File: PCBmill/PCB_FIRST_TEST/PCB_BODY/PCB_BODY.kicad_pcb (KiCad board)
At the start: 2 copper layers, 19 x 23.5 mm, 5 parts, among them U1 PC817

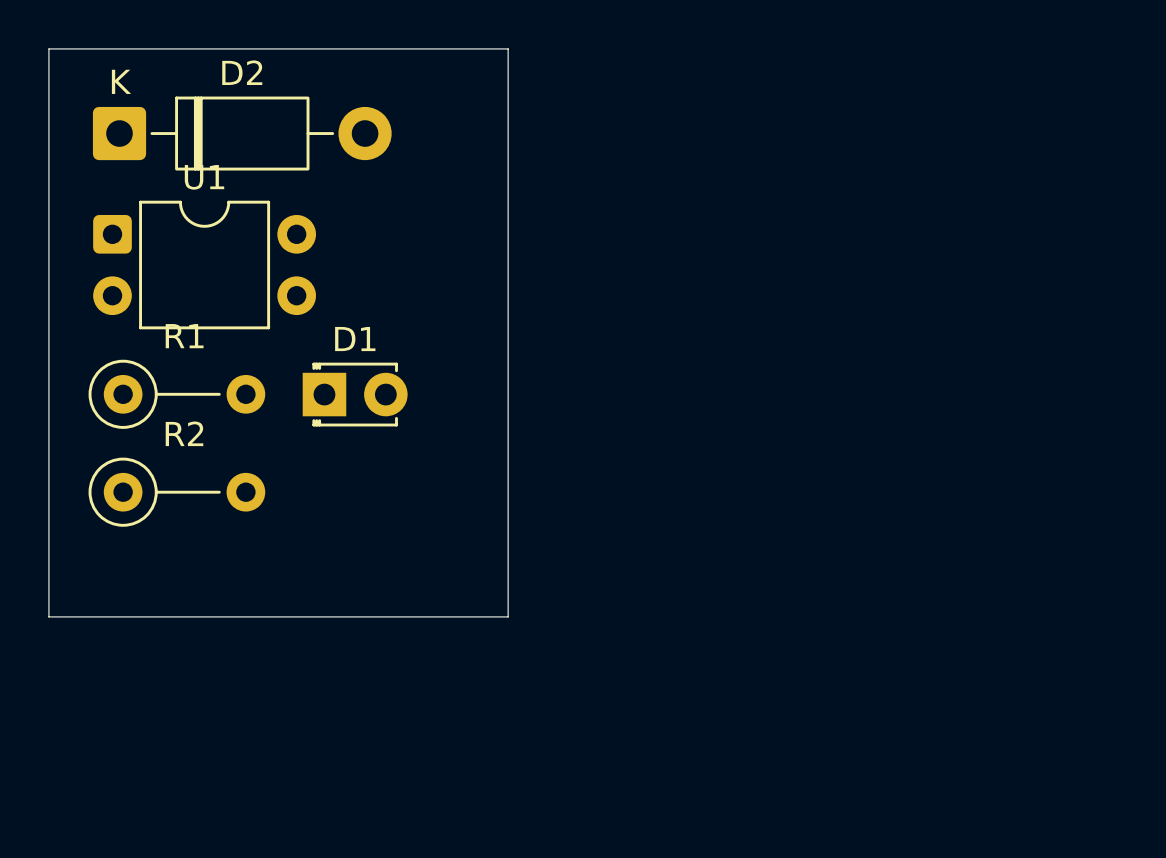
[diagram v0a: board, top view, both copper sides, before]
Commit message: added the thhings to the stuff
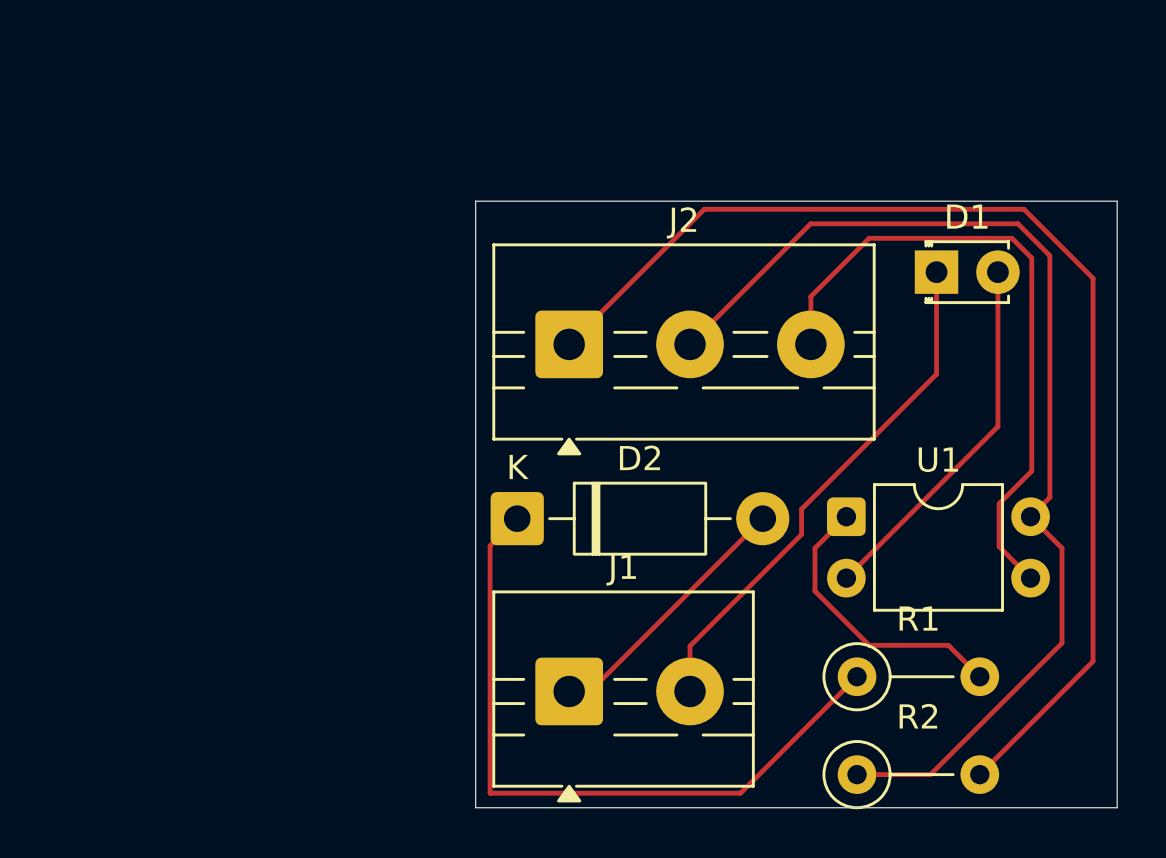
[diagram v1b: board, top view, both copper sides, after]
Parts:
- added J1: Screw_Terminal_01x02, TerminalBlock:TerminalBlock_MaiXu_MX126-5.0-02P_1x02_P5.00mm, F.Cu at (35.5, 41.1)
- added J2: Screw_Terminal_01x03, TerminalBlock:TerminalBlock_MaiXu_MX126-5.0-03P_1x03_P5.00mm, F.Cu at (35.5, 26.7)
- moved R1 32.5 mm to (47.4, 40.5)
- moved R2 32.5 mm to (47.4, 44.5)
- moved U1 32.5 mm to (47.0, 33.9)
- moved D1 25.8 mm to (50.7, 23.7)
- moved D2 22.9 mm to (33.4, 33.9)
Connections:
- D1 pad 1: GND -> Net-(D1-K)
- D2 pad 2: unconnected-(D2-A-Pad2) -> Net-(D2-A)
- R2 pad 2: +3.3V -> Net-(J2-Pin_1)
- U1 pad 1: Net-(D1-A) -> Net-(R1-Pad2)
- U1 pad 2: Net-(R1-Pad2) -> Net-(D1-A)
- U1 pad 3: GND -> Net-(J2-Pin_3)
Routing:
- net Net-(J2-Pin_1): track 0.00 -> 47.6 mm
- net Net-(J2-Pin_2): track 0.00 -> 45.1 mm
- net Net-(D2-K): track 0.00 -> 29.0 mm
- net Net-(J2-Pin_3): track 0.00 -> 26.8 mm
- net Net-(D1-K): track 0.00 -> 21.6 mm
- net Net-(D1-A): track 0.00 -> 15.3 mm
- net Net-(R1-Pad2): track 0.00 -> 11.9 mm
- net Net-(D2-A): track 0.00 -> 11.0 mm
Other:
- board size 19 x 23.5 mm -> 26.5 x 25.1 mm
